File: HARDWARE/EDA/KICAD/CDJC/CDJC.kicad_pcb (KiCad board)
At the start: 2 copper layers, 100 x 100 mm, 63 parts, among them J1 COM_IN, J2 COM_OUT, J3 POWER_IN, J4 POWER_OUT, J5 BIT_OUT, Q1 BC549, SW1 B-SET, U1 74LS04, U2 74LS32, U3 74LS08, U4 74LS08, U5 74LS08, U6 74LS08, U7 74LS32, U8 74LS32, U9 4017

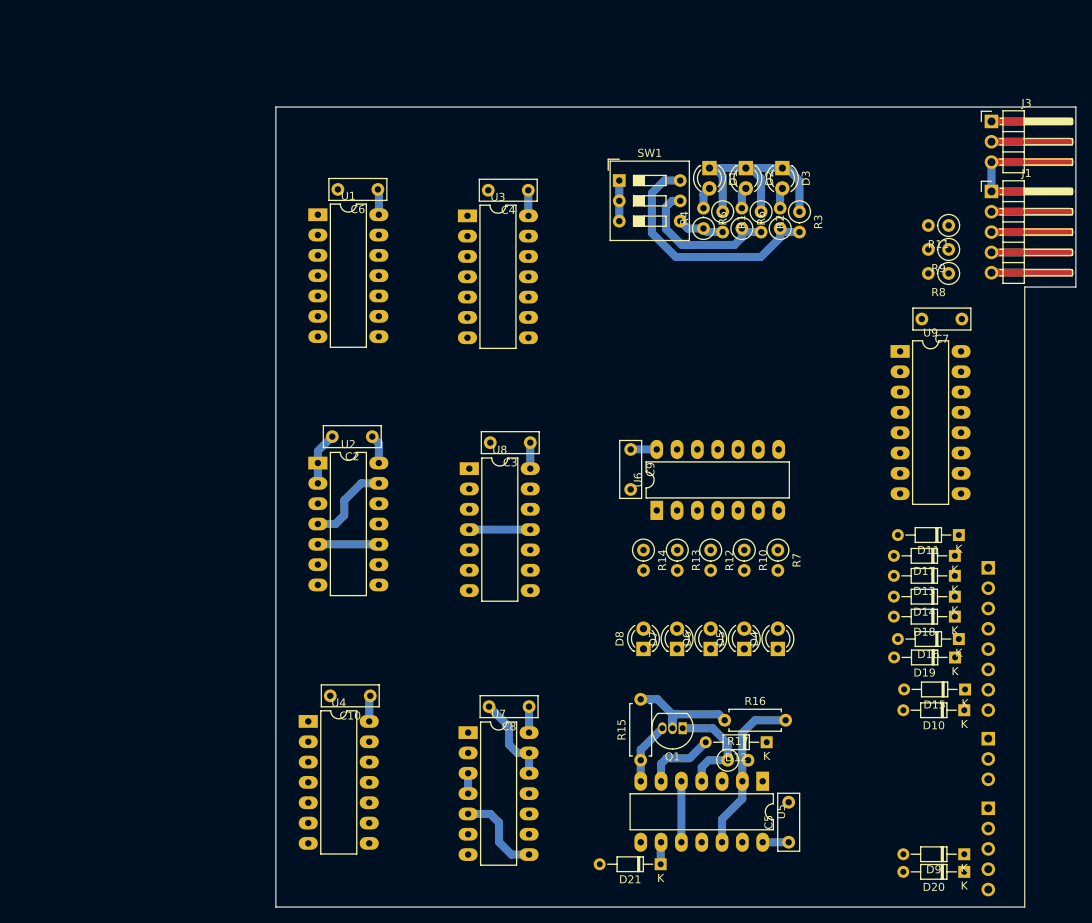
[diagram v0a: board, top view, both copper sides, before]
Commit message: stop work, go home
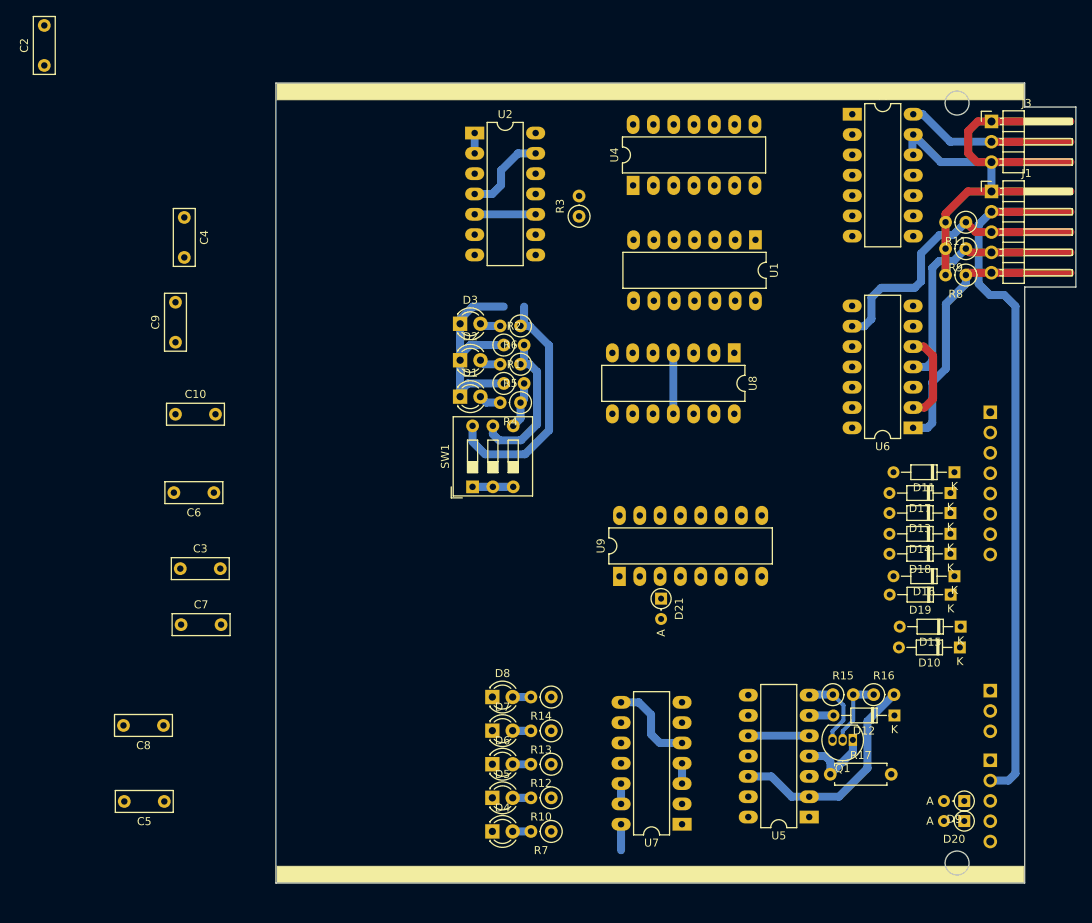
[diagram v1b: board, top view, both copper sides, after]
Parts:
- D20, D21, D9: footprint Diode_THT:D_DO-34_SOD68_P7.62mm_Horizontal -> Diode_THT:D_DO-34_SOD68_P2.54mm_Vertical_AnodeUp
- R15, R16: footprint Resistor_THT:R_Axial_DIN0207_L6.3mm_D2.5mm_P7.62mm_Horizontal -> Resistor_THT:R_Axial_DIN0207_L6.3mm_D2.5mm_P2.54mm_Vertical
- R17: footprint Resistor_THT:R_Axial_DIN0207_L6.3mm_D2.5mm_P2.54mm_Vertical -> Resistor_THT:R_Axial_DIN0207_L6.3mm_D2.5mm_P7.62mm_Horizontal
- moved C7 104.8 mm to (131.4, 114.2), turned to 0 degrees
- moved U4 78.3 mm to (187.9, 59.3), turned to 90 degrees
- moved C5 78.2 mm to (129.3, 136.3), turned to 180 degrees
- moved C2 61.9 mm to (114.3, 44.3), turned to 90 degrees
- moved C9 58.5 mm to (130.7, 78.9), turned to 90 degrees
- moved U1 54.8 mm to (203.2, 66.1), turned to 270 degrees
- moved U3 49.7 mm to (215.3, 50.4)
- moved C3 46.5 mm to (131.3, 107.2), turned to 0 degrees
- moved C8 45.8 mm to (129.2, 126.8)
- moved U2 45.7 mm to (168.1, 52.8)
- moved R7 45.2 mm to (177.7, 140.1), turned to 180 degrees
- moved U9 45.0 mm to (186.2, 108.2), turned to 90 degrees
- moved D3 44.7 mm to (166.3, 76.6), turned to 0 degrees
- moved C4 43.1 mm to (131.8, 63.3), turned to 270 degrees
- moved C6 43.1 mm to (135.5, 97.7)
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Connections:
- R9 pad 1: GNDD -> MRI
- R9 pad 2: MRI -> GNDD
- U6 pad 12: MRLMon -> Net-(D10-Pad1)
- U6 pad 13: Net-(D10-Pad1) -> MRLMon
- U6 pad 4: Net-(U6-Pad2) -> MRI
- U6 pad 5: MRI -> Net-(U6-Pad2)
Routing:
- net CLK: track 19.7 -> 97.1 mm
- net GNDD: track 117.6 -> 144.7 mm
- net LBLBI: track 19.7 -> 46.6 mm
- net EI: track 19.7 -> 46.0 mm
- net MRI: track 19.7 -> 42.7 mm
- net +5VD: track 51.1 -> 39.2 mm
- net Net-(U6-Pad2): track 0.00 -> 11.3 mm
- net Net-(D10-Pad1): track 20.8 -> 28.0 mm
- net Net-(Q1-Pad2): track 14.8 -> 8.83 mm
- net Net-(D12-Pad2): track 8.89 -> 3.03 mm
- net Net-(Q1-Pad1): track 13.9 -> 10.00 mm
- net Net-(D21-Pad1): track 2.77 -> 0.07 mm
- net Net-(D7-Pad2): track 0.00 -> 2.29 mm
- net Net-(D8-Pad2): track 0.00 -> 2.28 mm
- net Net-(D6-Pad2): track 0.00 -> 2.28 mm
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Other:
- outline, holes or cut-outs redrawn
